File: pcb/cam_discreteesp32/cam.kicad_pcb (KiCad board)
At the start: 4 copper layers, 75 x 65 mm, 116 parts, among them J1 Conn_Coaxial, J2 Power In, J3 PRGR, J4 Conn_01x24_Male, J5 SIM_Card, J6 Conn_Coaxial, J7 JTAG, Q1 IRLML6402, U1 TPS22810, U10 W25Q128JVS, U11 LY68L6400, U12 SRV05-4, U13 SIM800C, U2 FDC610, U3 XC6206-12, U4 XC6206-28, U5 LTC3103, U6 INA226, U7 ESP32-S2, U8 MP2307, Y1 32.768kHz, Y2 40Mhz

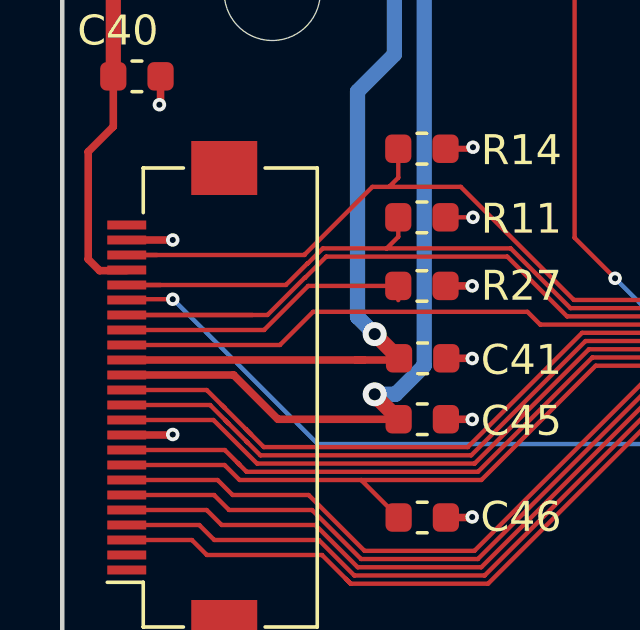
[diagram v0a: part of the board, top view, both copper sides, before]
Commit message: Small changes to pcb
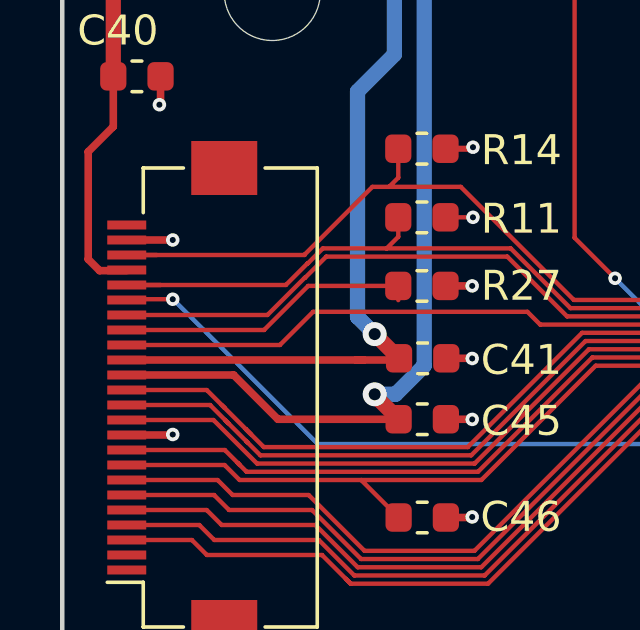
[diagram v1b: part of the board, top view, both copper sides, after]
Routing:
- net CSI_VSYNC: track 34.7 -> 30.5 mm
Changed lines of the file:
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@@
     (thickness 1.6)
     (drawings 29)
-    (tracks 1279)
+    (tracks 1278)
     (zones 0)
     (modules 116)
@@
   (segment (start 137.211 83.5595) (end 136.4063 83.5595) (width 0.146812) (layer F.Cu) (net 31))
   (segment (start 136.2548 83.5491) (end 136.3959 83.5491) (width 0.146812) (layer F.Cu) (net 31))
-  (segment (start 102.15 82.25) (end 106.345 82.25) (width 0.146812) (layer F.Cu) (net 32))
   (segment (start 108.084335 81.006177) (end 108.096823 81.006177) (width 0.146812) (layer F.Cu) (net 32))
   (segment (start 129.7798 80.3116) (end 130.2173 80.3116) (width 0.146812) (layer F.Cu) (net 32))
